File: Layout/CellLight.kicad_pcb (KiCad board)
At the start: 2 copper layers, 58.4 x 48.3 mm, 42 parts, among them J1 Conn_01x03, J2 Conn_01x03, J3 Conn_01x03, J4 Conn_01x06, J5 COMM, J6 I2C, SW1 SW_Push, U1 DSPIC33FJ128MC804, U2 TS3A4751PWR, U3 MB85RC256, U4 TPS562200, U5 AP2112K-3.3, U6 SN74LVC1T45DCK

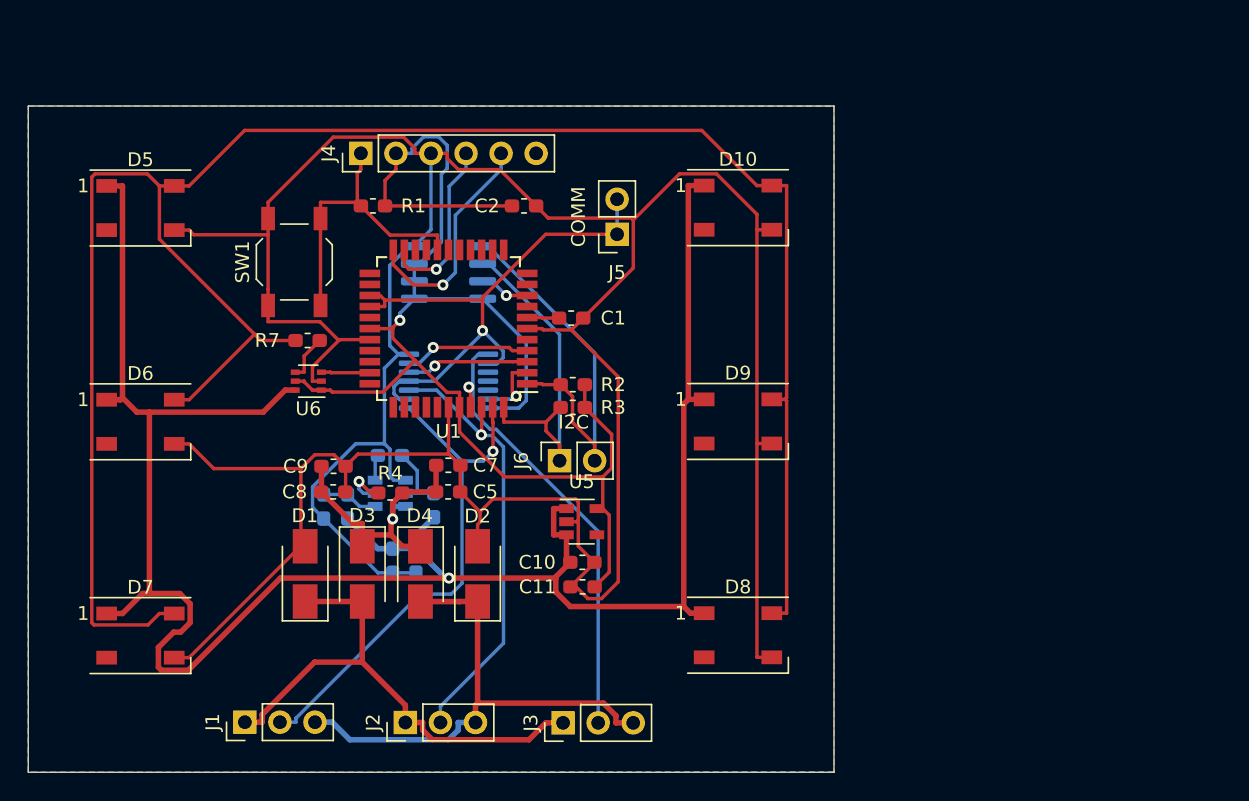
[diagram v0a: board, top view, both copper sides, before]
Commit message: Layout
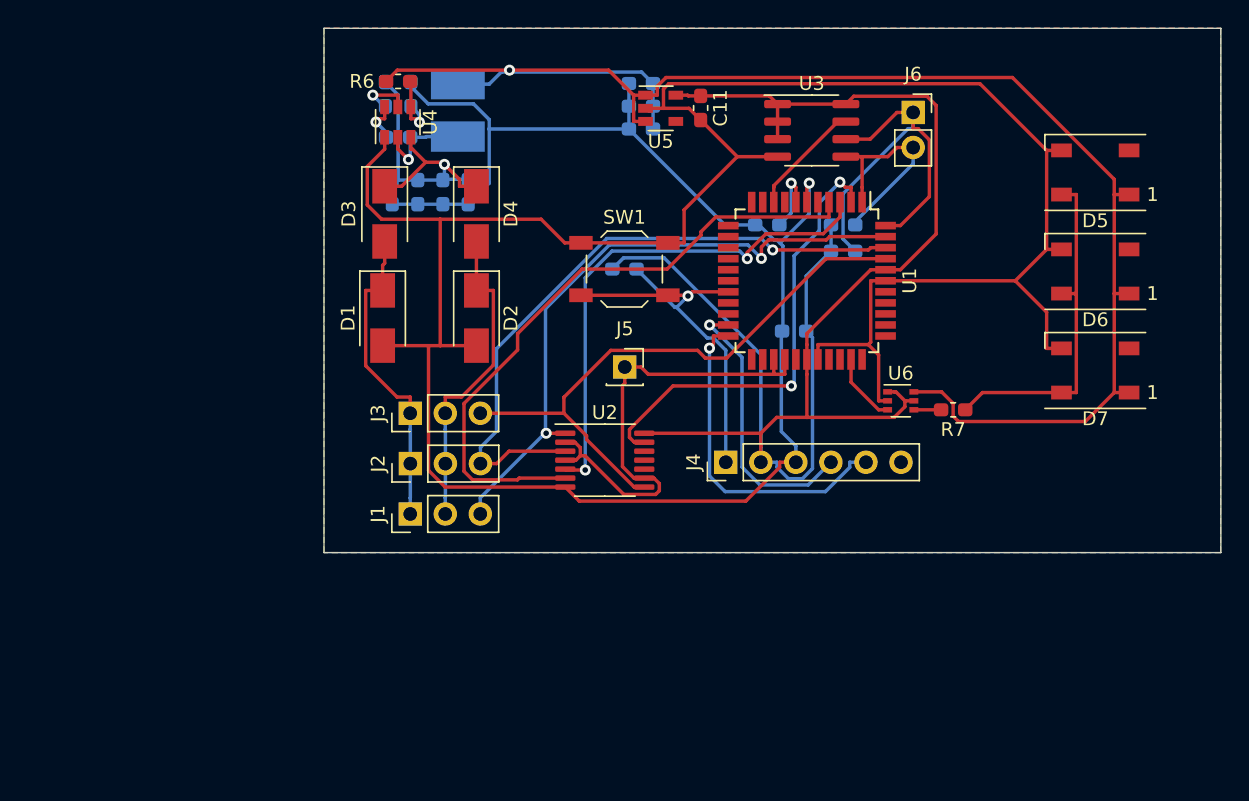
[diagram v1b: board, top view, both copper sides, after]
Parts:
- removed D10, D8, D9: WS2812B, LED_SMD:LED_WS2812B_PLCC4_5.0x5.0mm_P3.2mm
- C1, C10, C2, C5, C7, C8, C9, R1, R2, R3, R4: moved to B.Cu
- J5: value COMM -> Conn_01x01_Female; footprint Connector_PinSocket_2.54mm:PinSocket_1x02_P2.54mm_Vertical -> Connector_PinSocket_2.54mm:PinSocket_1x01_P2.54mm_Vertical
- J6: value I2C -> Conn_01x02_Female
- L1: footprint Inductor_SMD:L_0603_1608Metric_Pad1.05x0.95mm_HandSolder -> Inductor_SMD:L_Taiyo-Yuden_NR-40xx_HandSoldering
- R6, U2, U3, U4: moved to F.Cu
- moved D7 71.8 mm to (237.3, 118.2), turned to 180 degrees
- moved D6 70.1 mm to (237.3, 111.0), turned to 180 degrees
- moved D5 69.2 mm to (237.3, 103.8), turned to 180 degrees
- moved R7 47.1 mm to (227.1, 121.0), turned to 180 degrees
- moved U6 43.0 mm to (223.2, 120.4), turned to 0 degrees
- moved C4 38.2 mm to (204.4, 97.4), turned to 180 degrees
- moved C6 37.5 mm to (204.4, 99.0), turned to 180 degrees
- moved J6 36.0 mm to (224.2, 99.5), turned to 0 degrees
- moved C11 35.7 mm to (208.8, 99.2), turned to 270 degrees
- moved J4 34.6 mm to (210.6, 124.8)
- moved C10 31.7 mm to (204.4, 100.7), turned to 180 degrees
- moved R6 31.0 mm to (186.8, 97.2), turned to 180 degrees
- moved R5 30.5 mm to (187.8, 98.2), turned to 90 degrees
- moved U5 30.5 mm to (205.8, 99.2)
- moved R4 28.9 mm to (185.9, 98.2), turned to 90 degrees
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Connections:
- J1 pad 2: PORT1_IO -> PRI_LO
- J1 pad 3: PRI_LO -> PORT1_IO
- J2 pad 2: PORT2_IO -> PRI_LO
- J2 pad 3: PRI_LO -> PORT2_IO
- J3 pad 2: PORT3_IO -> PRI_LO
- J3 pad 3: PRI_LO -> PORT3_IO
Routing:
- net Net-(D10-Pad4): track 150.5 -> 25.1 mm
- net +5V: track 153.7 -> 114.4 mm
- net PORT3_SEL: track 9.21 -> 46.5 mm, vias 1 -> 0
- net PORT2_SEL: track 8.88 -> 37.5 mm, vias 1 -> 2
- net PORT1_SEL: track 5.03 -> 33.1 mm, vias 1 -> 2
- net +3V3: track 100.0 -> 119.5 mm, vias 1 -> 0
- net PRI_LO: track 38.1 -> 23.1 mm
- net PORT2_IO: track 32.4 -> 47.2 mm
- net PRI_HI: track 37.6 -> 22.9 mm
- net SDA: track 28.1 -> 15.8 mm
- net PORT3_IO: track 33.4 -> 43.3 mm, vias 1 -> 0
- net GND: track 257.3 -> 248.2 mm, vias 0 -> 1
- net PORT1_IO: track 37.6 -> 46.4 mm, vias 1 -> 2
- net PGEC: track 16.6 -> 24.2 mm
- net PGED: track 12.8 -> 20.3 mm
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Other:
- board size 58.4 x 48.3 mm -> 65 x 38 mm
